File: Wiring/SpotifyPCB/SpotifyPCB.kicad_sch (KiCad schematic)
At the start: 3 parts, among them SW1 RotaryEncoder_Switch, U1 ESP32-S3, U2 ST7735

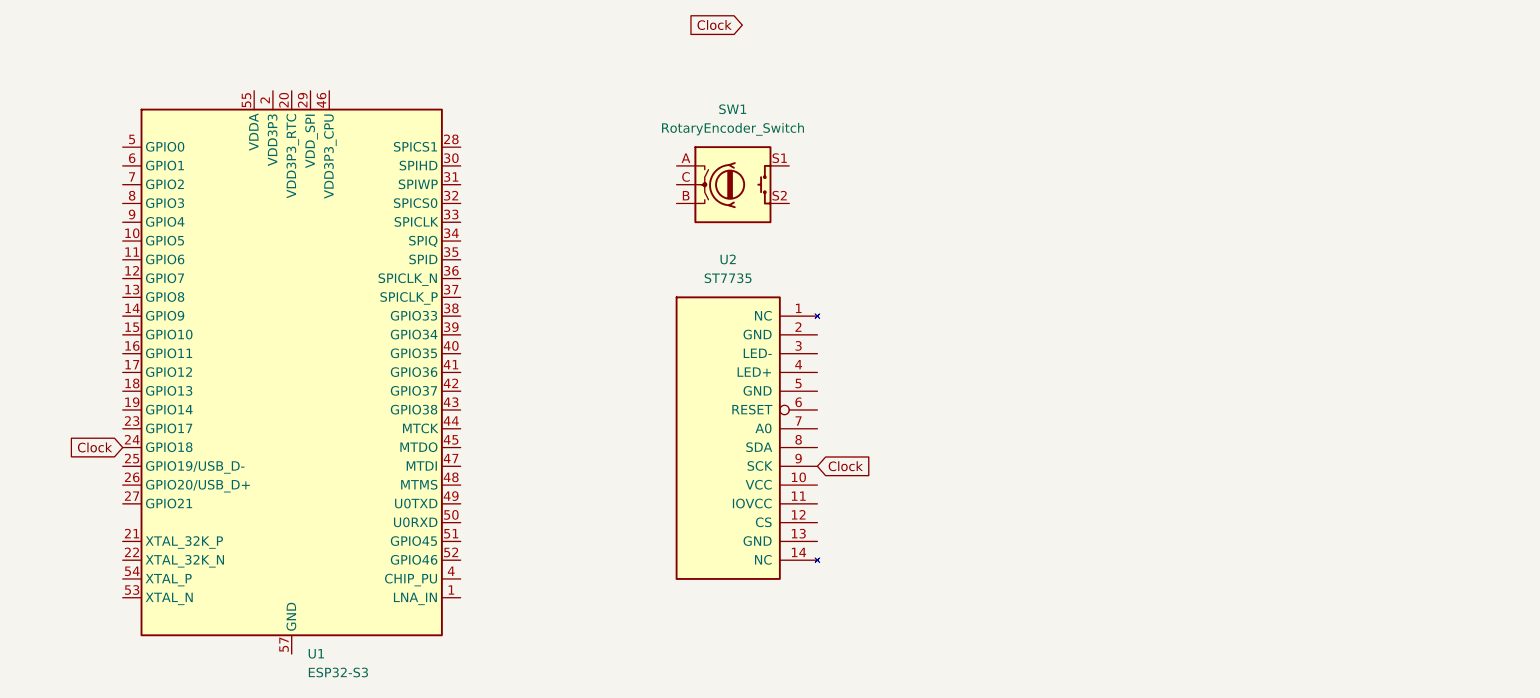
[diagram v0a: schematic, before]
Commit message: Wiring
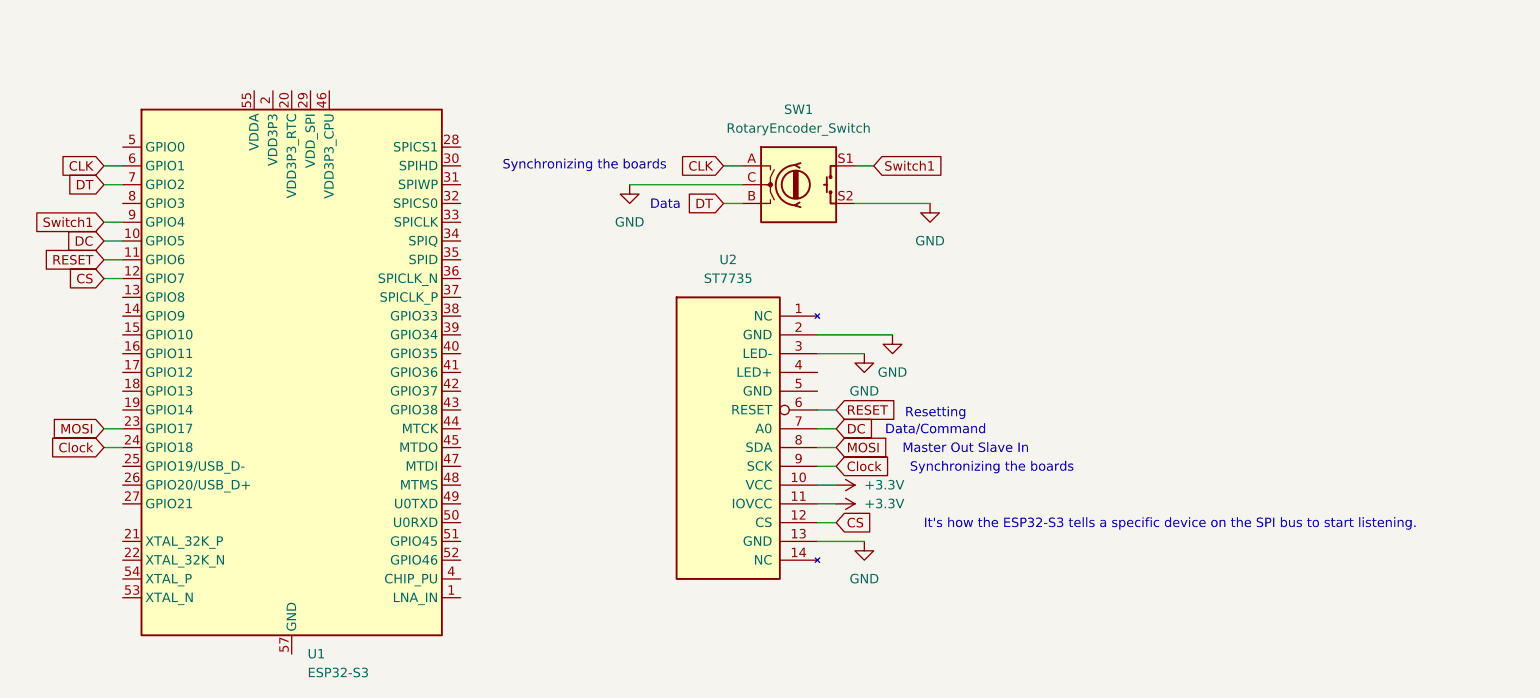
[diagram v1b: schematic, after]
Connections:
- net +3.3V: now reaches U2.10 (VCC)
- net +3.3V: now also U2.11 (IOVCC)
- net CS: now reaches U2.12 (CS)
- net CS: now also U1.12 (GPIO7)
- net GND: now reaches U2.13 (GND)
- net GND: now also SW1.C, SW1.S2, U2.2 (GND), U2.3 (LED-)
- net RESET: now reaches U2.6 (RESET)
- net RESET: now also U1.11 (GPIO6)
- net DC: now reaches U2.7 (A0)
- net DC: now also U1.10 (GPIO5)
- net MOSI: now reaches U2.8 (SDA)
- net MOSI: now also U1.23 (GPIO17)
- net CLK: now reaches SW1.A
- net CLK: now also U1.6 (GPIO1)
- net DT: now reaches SW1.B
- net DT: now also U1.7 (GPIO2)
- net Switch1: now reaches SW1.S1
- net Switch1: now also U1.9 (GPIO4)
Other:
- note added: "Data"
- note added: "Data/Command"
- note added: "It's how the ESP32-S3 tells a specific device on the SPI bus to start listening."
- note added: "Master Out Slave In"
- note added: "Resetting"
- note added: "Synchronizing the boards"
- moved on the sheet: SW1

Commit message: Wiring
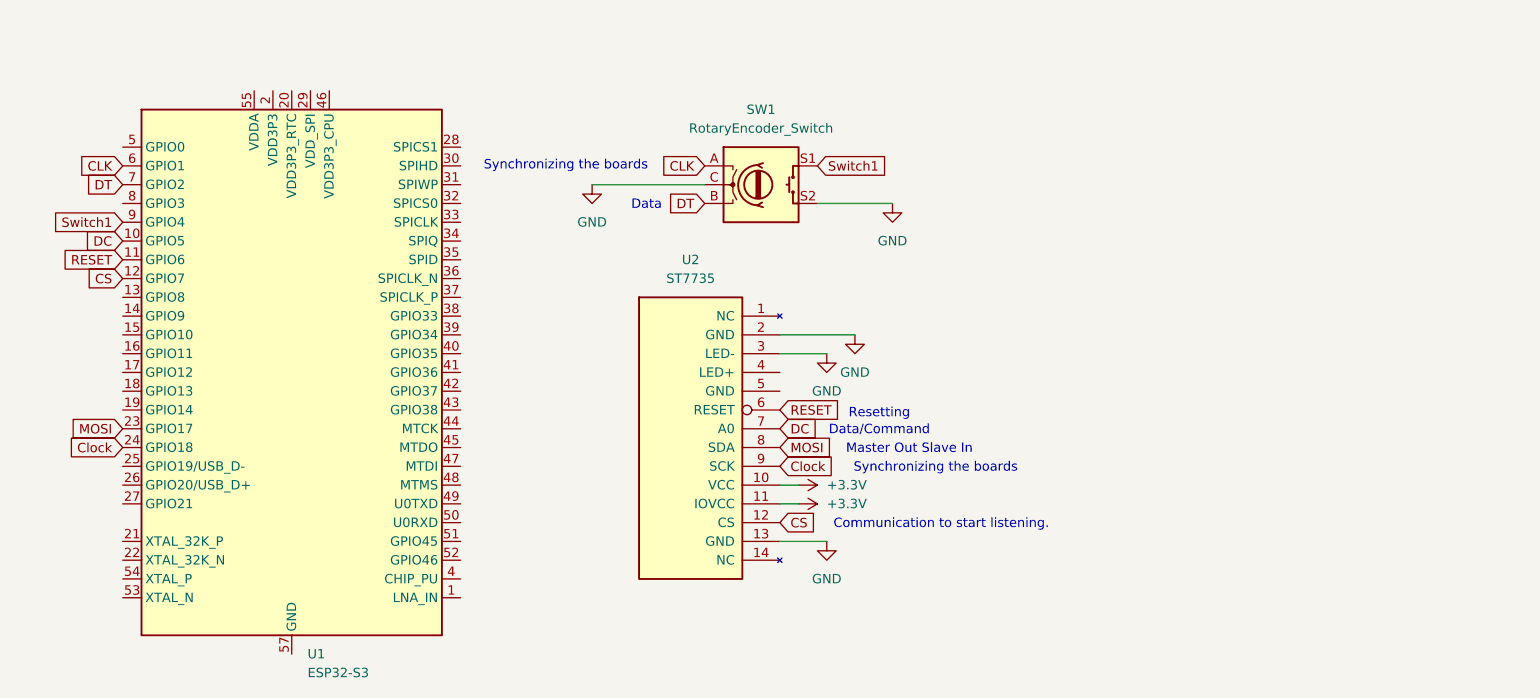
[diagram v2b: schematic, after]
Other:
- note added: "Communication to start listening."
- note removed: "It's how the ESP32-S3 tells a specific device on the SPI bus to start listening."
- moved on the sheet: SW1, U2
